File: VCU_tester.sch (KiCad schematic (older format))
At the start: 40 parts, among them J1 Conn_01x04_Male, J12 Conn_01x08_Male, J13 Conn_01x08_Male, J14 USB_C_Receptacle, J15 USB_B_Micro, J2 Screw_Terminal_01x02, J500 Conn_01x10_Female, J501 Conn_01x08_Female, J502 Conn_01x08_Female, J503 Conn_01x08_Female, J504 Conn_01x08_Female, J505 Conn_01x08_Female, J507 Conn_02x18_Odd_Even, J7 Conn_01x04_Male, P8 BeagleBone_Black_Header, P9 BeagleBone_Black_Header, U1 REF3020, U6 DS3231MZ, U7 DS3231MZ

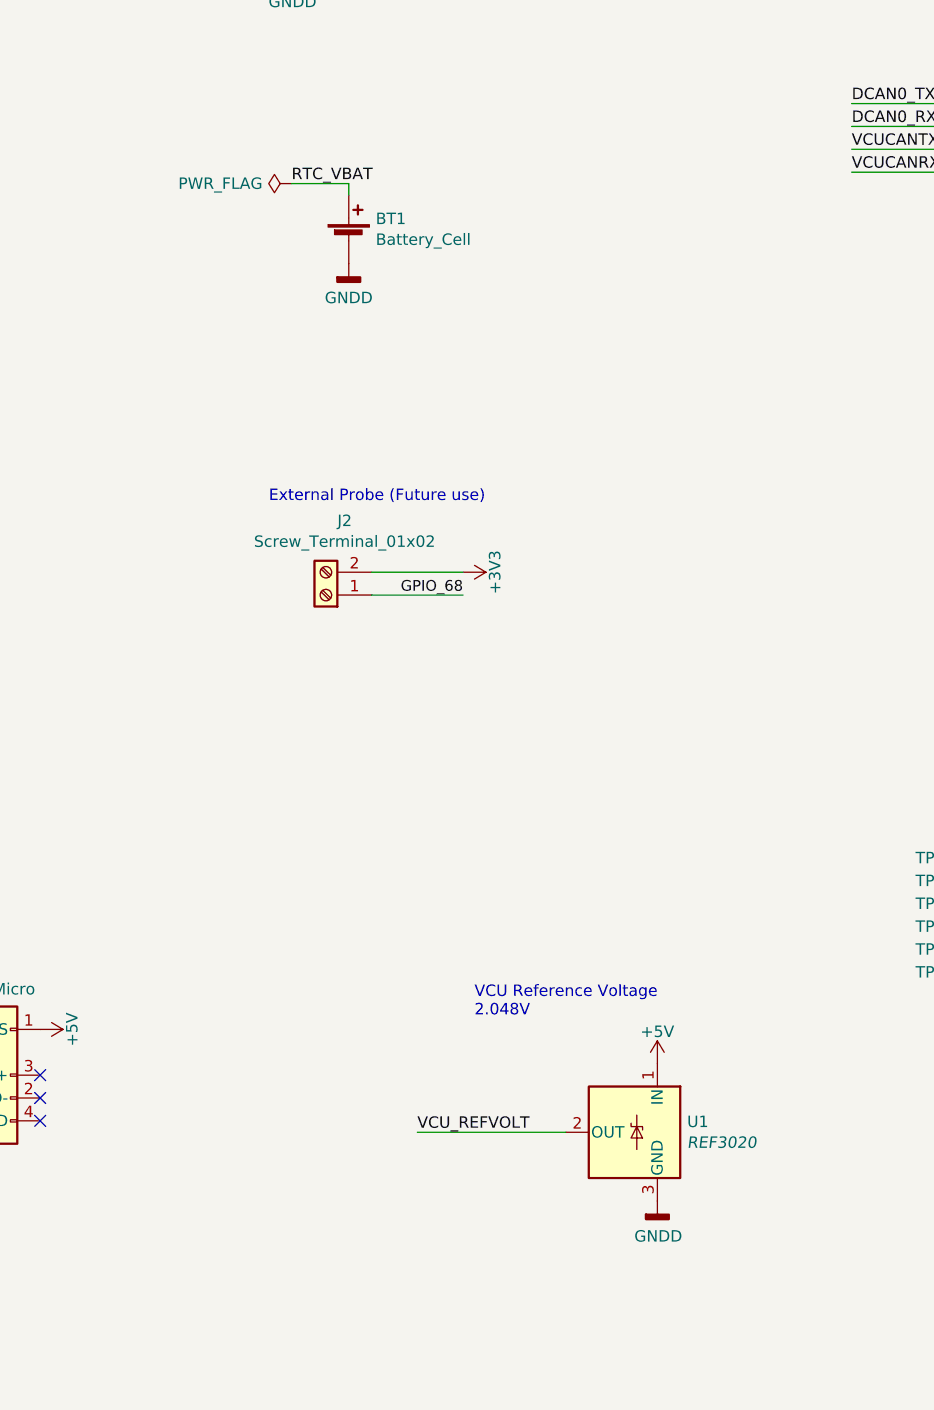
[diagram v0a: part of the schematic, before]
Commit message: new, compact (and sexy) design
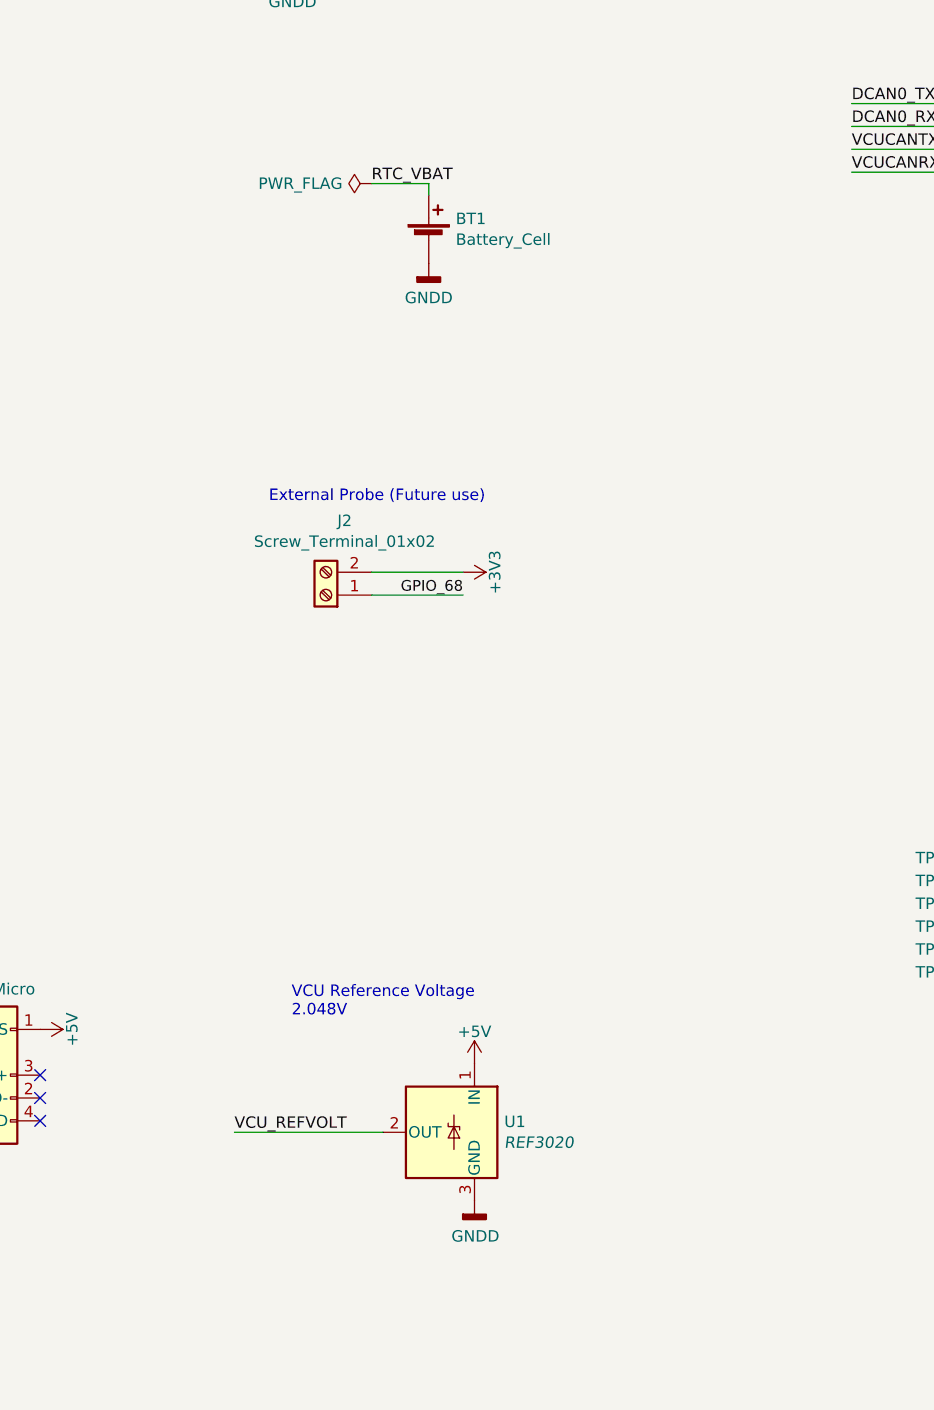
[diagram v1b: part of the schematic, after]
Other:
- moved on the sheet: BT1, U1
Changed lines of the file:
@@
 RTC VCU
 Wire Wire Line
-	10750 8450 11400 8450
-Text Label 10750 8450 0    50   ~ 0
+	9950 8450 10600 8450
+Text Label 9950 8450 0    50   ~ 0
 VCU_REFVOLT
 $Comp
 L Reference_Voltage:REF3020 U1
 U 1 1 5F9A6E14
-P 11700 8450
-F 0 "U1" H 11470 8496 50  0000 R CNN
-F 1 "REF3020" H 11470 8405 50  0000 R CIN
-F 2 "Package_TO_SOT_SMD:SOT-23" H 11700 8000 50  0001 C CIN
-F 3 "http://www.ti.com/lit/ds/symlink/ref3033.pdf" H 11800 8100 50  0001 C CIN
-F 4 "296-26321-1-ND" H 11700 8450 50  0001 C CNN "Part"
-	1    11700 8450
+P 10900 8450
+F 0 "U1" H 10670 8496 50  0000 R CNN
+F 1 "REF3020" H 10670 8405 50  0000 R CIN
+F 2 "Package_TO_SOT_SMD:SOT-23" H 10900 8000 50  0001 C CIN
+F 3 "http://www.ti.com/lit/ds/symlink/ref3033.pdf" H 11000 8100 50  0001 C CIN
+F 4 "296-26321-1-ND" H 10900 8450 50  0001 C CNN "Part"
+	1    10900 8450
 	-1   0    0    -1
 $EndComp
@@
 L power:GNDD #PWR0104
 U 1 1 5F9A8026
-P 11800 8750
-F 0 "#PWR0104" H 11800 8500 50  0001 C CNN
-F 1 "GNDD" H 11804 8595 50  0000 C CNN
-F 2 "" H 11800 8750 50  0001 C CNN
-F 3 "" H 11800 8750 50  0001 C CNN
-	1    11800 8750
+P 11000 8750
+F 0 "#PWR0104" H 11000 8500 50  0001 C CNN
+F 1 "GNDD" H 11004 8595 50  0000 C CNN
+F 2 "" H 11000 8750 50  0001 C CNN
+F 3 "" H 11000 8750 50  0001 C CNN
+	1    11000 8750
 	1    0    0    -1
 $EndComp
@@
 L power:+5V #PWR0105
 U 1 1 5F9AA125
-P 11800 8150
-F 0 "#PWR0105" H 11800 8000 50  0001 C CNN
-F 1 "+5V" H 11800 8290 50  0000 C CNN
-F 2 "" H 11800 8150 60  0000 C CNN
-F 3 "" H 11800 8150 60  0000 C CNN
-	1    11800 8150
-	1    0    0    -1
-$EndComp
-Text Notes 11000 7950 0    50   ~ 0
+P 11000 8150
+F 0 "#PWR0105" H 11000 8000 50  0001 C CNN
+F 1 "+5V" H 11000 8290 50  0000 C CNN
+F 2 "" H 11000 8150 60  0000 C CNN
+F 3 "" H 11000 8150 60  0000 C CNN
+	1    11000 8150
+	1    0    0    -1
+$EndComp
+Text Notes 10200 7950 0    50   ~ 0
 VCU Reference Voltage\n2.048V
 $Comp
@@
 L Device:Battery_Cell BT1
 U 1 1 601EDE3A
-P 10450 4550
-F 0 "BT1" H 10568 4646 50  0000 L CNN
-F 1 "Battery_Cell" H 10568 4555 50  0000 L CNN
-F 2 "Battery:BatteryHolder_MPD_BC2003_1x2032" V 10450 4610 50  0001 C CNN
-F 3 "~" V 10450 4610 50  0001 C CNN
-F 4 "BU2032SM-FH-GCT-ND" H 10450 4550 50  0001 C CNN "Part"
-	1    10450 4550
+P 10800 4550
+F 0 "BT1" H 10918 4646 50  0000 L CNN
+F 1 "Battery_Cell" H 10918 4555 50  0000 L CNN
+F 2 "Battery:BatteryHolder_MPD_BC2003_1x2032" V 10800 4610 50  0001 C CNN
+F 3 "~" V 10800 4610 50  0001 C CNN
+F 4 "BU2032SM-FH-GCT-ND" H 10800 4550 50  0001 C CNN "Part"
+	1    10800 4550
 	1    0    0    -1
 $EndComp
@@
 L power:GNDD #PWR018
 U 1 1 602101F4
-P 10450 4650
-F 0 "#PWR018" H 10450 4400 50  0001 C CNN
-F 1 "GNDD" H 10450 4500 50  0000 C CNN
-F 2 "" H 10450 4650 60  0000 C CNN
-F 3 "" H 10450 4650 60  0000 C CNN
-	1    10450 4650
-	1    0    0    -1
-$EndComp
-Wire Wire Line
-	10450 4350 10450 4300
-Wire Wire Line
-	10450 4300 10200 4300
-Text Label 10200 4300 0    50   ~ 0
+P 10800 4650
+F 0 "#PWR018" H 10800 4400 50  0001 C CNN
+F 1 "GNDD" H 10800 4500 50  0000 C CNN
+F 2 "" H 10800 4650 60  0000 C CNN
+F 3 "" H 10800 4650 60  0000 C CNN
+	1    10800 4650
+	1    0    0    -1
+$EndComp
+Wire Wire Line
+	10800 4350 10800 4300
+Wire Wire Line
+	10800 4300 10550 4300
+Text Label 10550 4300 0    50   ~ 0
 RTC_VBAT
 Text Label 7950 3600 1    50   ~ 0
@@
 L power:PWR_FLAG #FLG0108
 U 1 1 6081FF4F
-P 10200 4300
-F 0 "#FLG0108" H 10200 4375 50  0001 C CNN
-F 1 "PWR_FLAG" V 10200 4427 50  0000 L CNN
-F 2 "" H 10200 4300 50  0001 C CNN
-F 3 "~" H 10200 4300 50  0001 C CNN
-	1    10200 4300
+P 10550 4300
+F 0 "#FLG0108" H 10550 4375 50  0001 C CNN
+F 1 "PWR_FLAG" V 10550 4427 50  0000 L CNN
+F 2 "" H 10550 4300 50  0001 C CNN
+F 3 "~" H 10550 4300 50  0001 C CNN
+	1    10550 4300
 	0    -1   -1   0
 $EndComp
